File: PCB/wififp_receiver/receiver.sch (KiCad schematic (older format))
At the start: 17 parts, among them IC1 ATTINY2313-P, P1 ICISP1, P2 USB, U1 rf-receiver, X1 12MHz

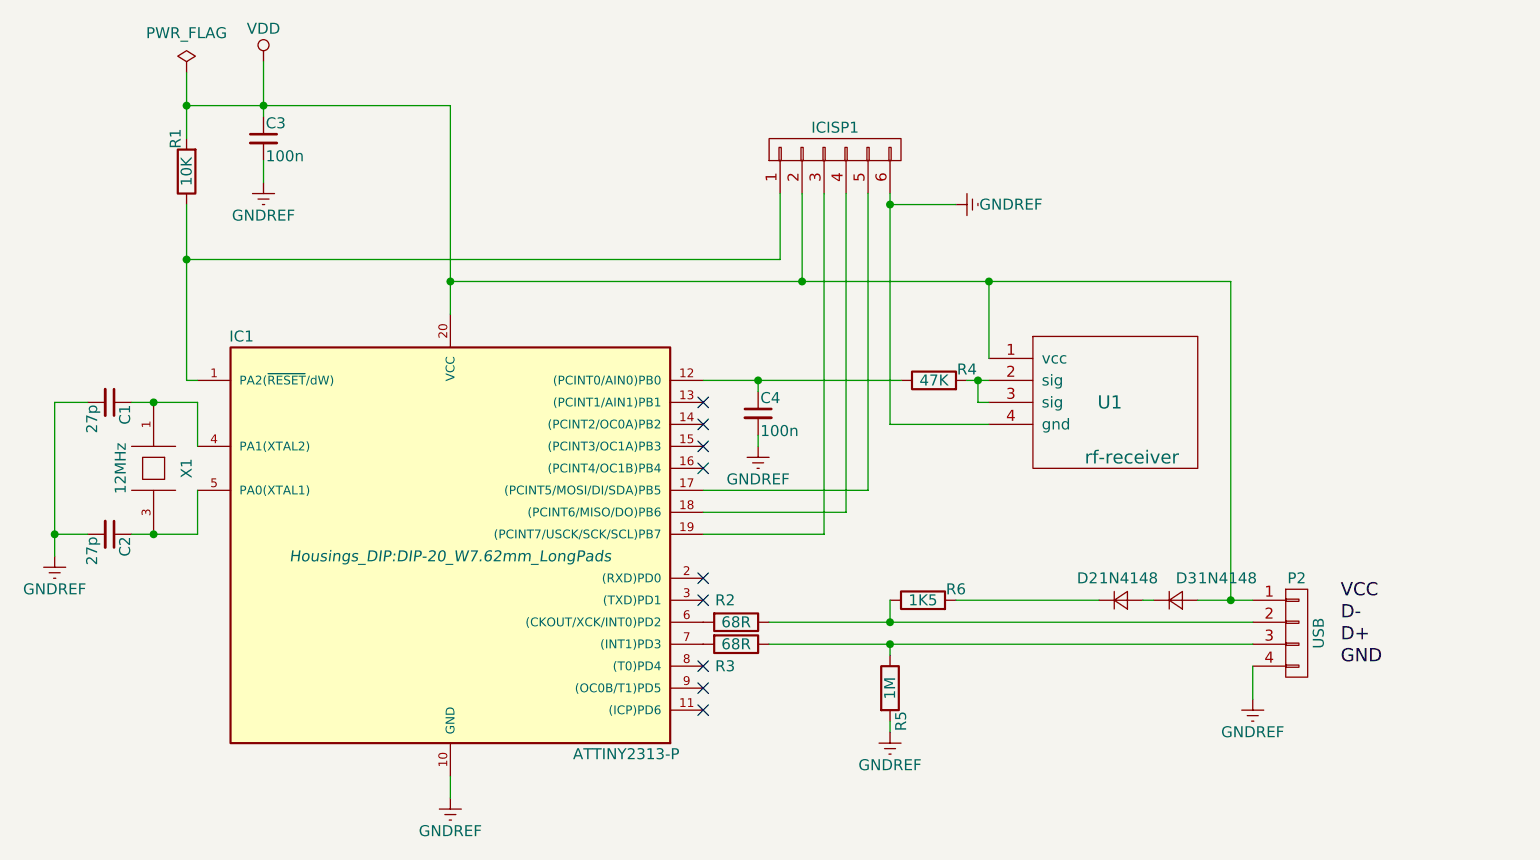
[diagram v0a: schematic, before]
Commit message: Updated the schematic
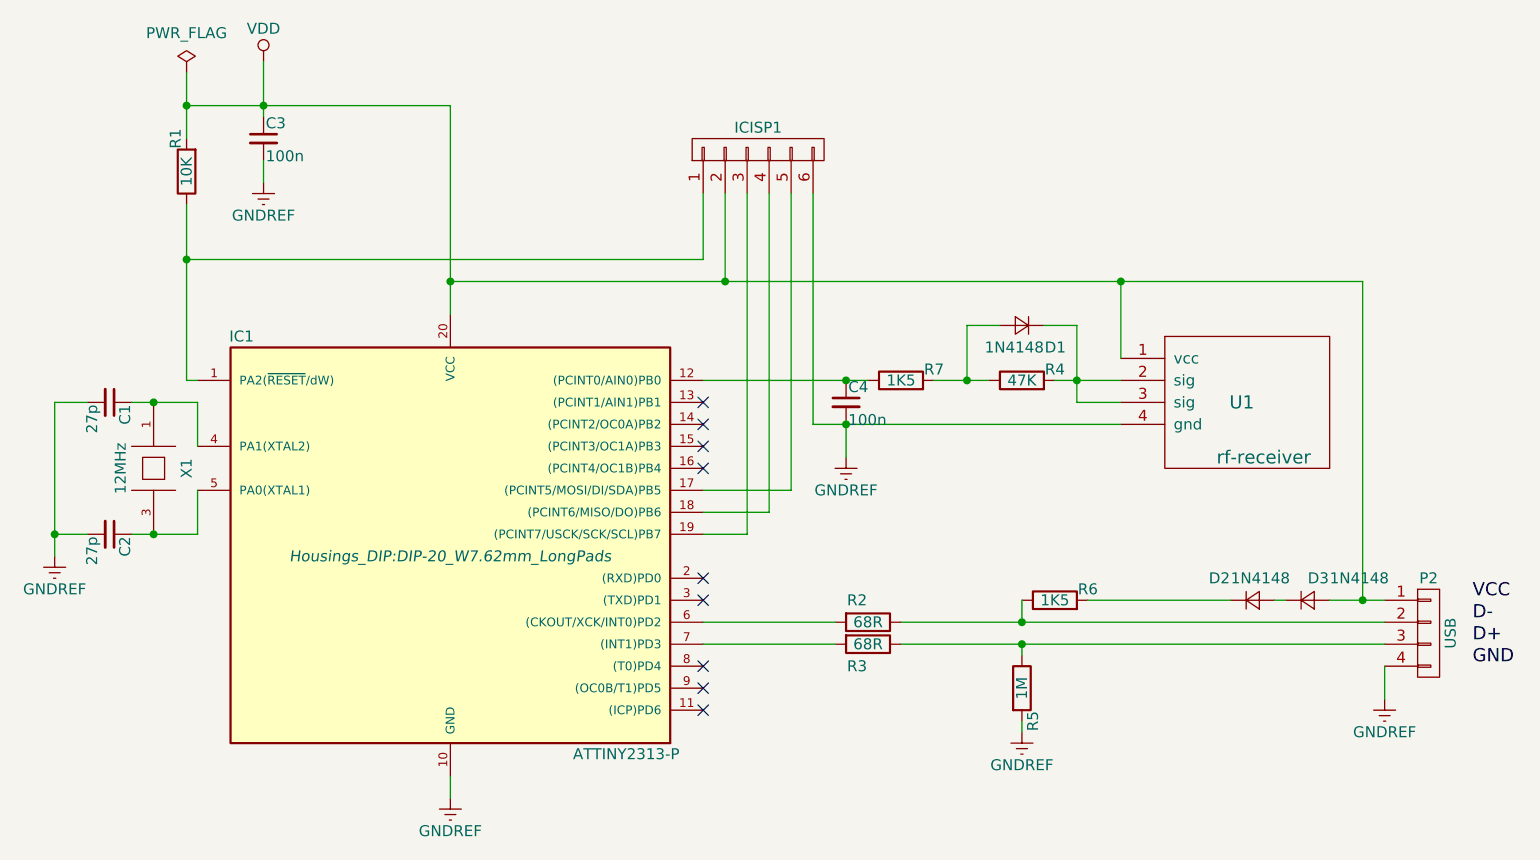
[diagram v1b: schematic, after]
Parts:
- added D1: 1N4148, Diodes_SMD:D_0805, symbol D_Small
- added R7: 1K5, Capacitors_SMD:C_0805_HandSoldering, symbol R
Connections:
- net at C4.1, IC1.12 ((PCINT0/AIN0)PB0): now also R7.1; no longer R4.1
- net at R4.2, U1.2 (sig), U1.3 (sig): now also D1.1 (K)
- new net: D1.2 (A), R4.1, R7.2
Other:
- moved on the sheet: C4, D2, D3, P2, R2, R3, R4, R5, R6, U1
